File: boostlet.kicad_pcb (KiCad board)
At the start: 2 copper layers, 40 x 35 mm, 53 parts, among them J1 Conn_01x13_Socket, J2 Conn_01x05_Socket, J3 Conn_01x05_Socket, Q1 BSS138, Q2 BSS138, U1 PAM2401, U2 AP2112K-3.3

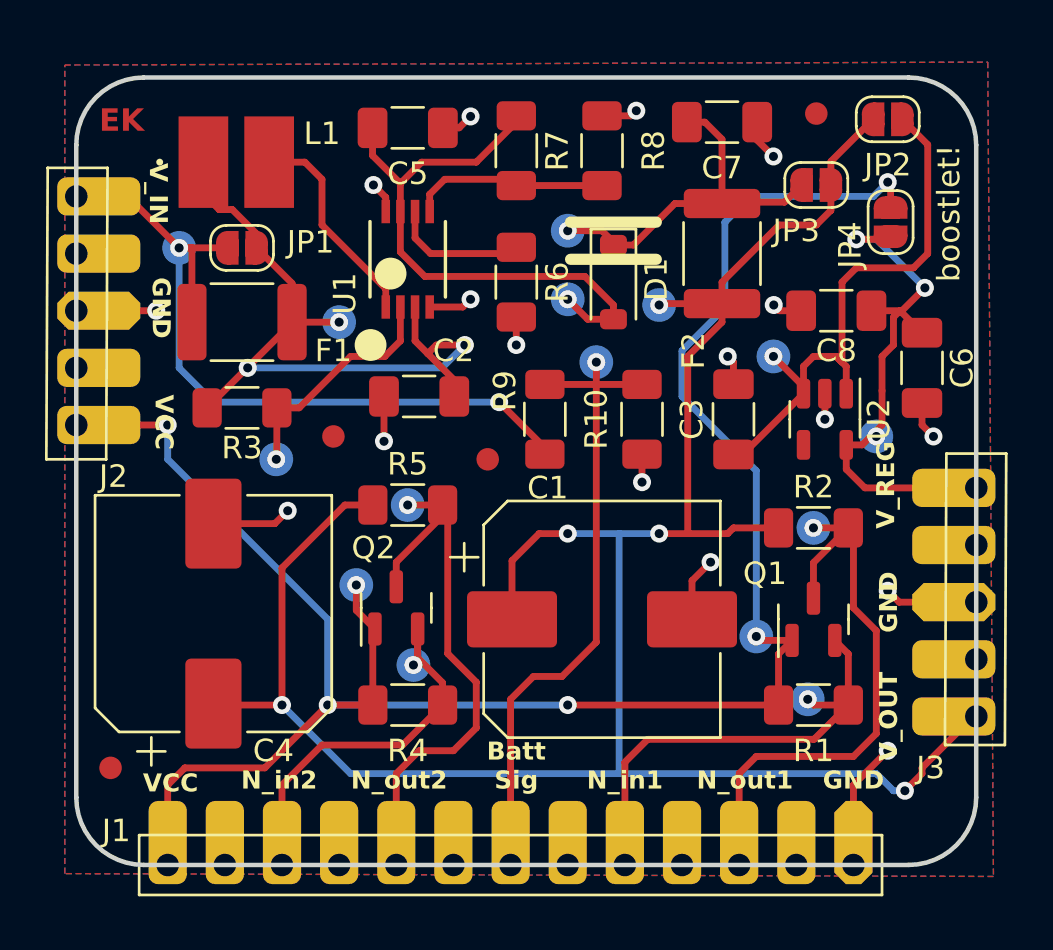
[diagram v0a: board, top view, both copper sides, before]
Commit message: Version 1.2
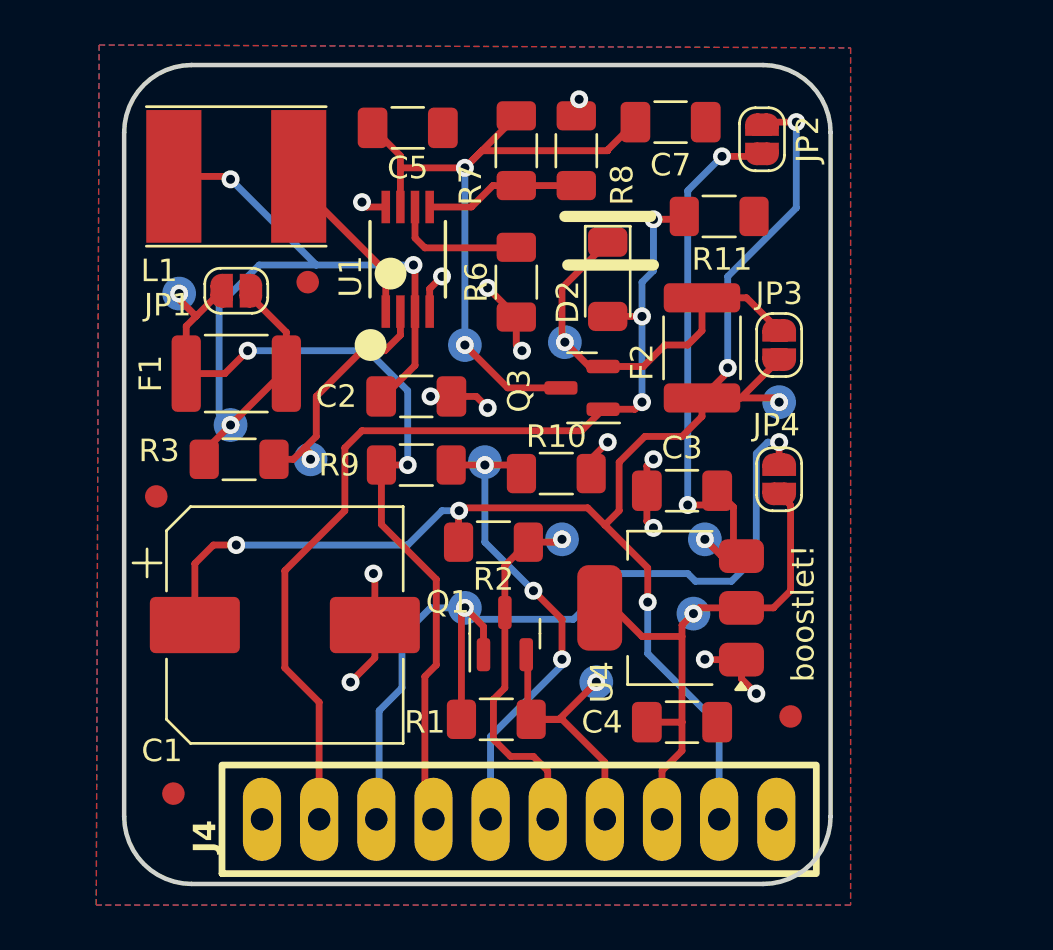
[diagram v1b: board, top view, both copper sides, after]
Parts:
- removed the C4 at (109.7, 103.6)
- removed C6: 4.7 uF, Capacitor_SMD:C_1206_3216Metric_Pad1.33x1.80mm_HandSolder
- removed D1: D_Schottky 3A, Diode_SMD:D_SOD-123
- removed J1: Conn_01x13_Socket, !EK_Library:Castellated_1x13_P2.54mm
- removed J2, J3: Conn_01x05_Socket, !EK_Library:Castellated_1x05_P2.54mm
- removed Q2: BSS138, Package_TO_SOT_SMD:SOT-23
- removed R4, R5: 10k, Resistor_SMD:R_1206_3216Metric_Pad1.30x1.75mm_HandSolder
- removed TP10, TP8, TP9: TestPoint, TestPoint:TestPoint_Pad_D1.5mm
- removed U2: AP2112K-3.3, Package_TO_SOT_SMD:SOT-23-5
- added D2: PMEG40T30ERX 40V 3A, Diode_SMD:D_SOD-123, F.Cu at (127.3, 88.8)
- added J4: Conn_01x10_Socket, !RobotButterfly:Oval_1x10_P2.54mm, F.Cu at (111.9, 112.8)
- added Q3: DMG3415U, Package_TO_SOT_SMD:SOT-23, F.Cu at (126.1, 93.6)
- added R11: 100k, Resistor_SMD:R_1206_3216Metric_Pad1.30x1.75mm_HandSolder, F.Cu at (132.2, 86.0)
- added U4: AP2111H-3.3TRG1, Package_TO_SOT_SMD:SOT-223-3_TabPin2, F.Cu at (130.0, 103.4)
- C1: value 680 uF @ 10 V -> 1000 uF @ 16 V
- C3: value 4.7 uF -> 1 uF
- L1: value 2.2 uH, 3 A -> 4.7 uH, 3 A; footprint !EK_Library:INDUCTOR_IND_IFSC_1515AH_VIS-M -> Inductor_SMD:L_Taiyo-Yuden_NR-60xx_HandSoldering
- moved FID3 26.8 mm to (135.4, 108.2)
- moved C4 19.5 mm to (130.6, 108.5), turned to 0 degrees
- moved FID4 14.8 mm to (107.2, 98.4)
- moved R2 14.2 mm to (122.2, 100.5)
- moved R1 14.1 mm to (122.3, 108.3)
- moved C1 14.1 mm to (112.9, 104.1)
- moved Q1 13.7 mm to (122.7, 104.5)
- moved TP2 13.0 mm to (120.9, 103.4)
- moved JP4 12.5 mm to (134.9, 97.7)
- moved TP13 11.3 mm to (131.1, 103.6)
- moved TP5 11.2 mm to (125.2, 100.3)
- moved TP1 9.43 mm to (126.7, 106.7)
- moved TP11 8.68 mm to (131.6, 100.3)
- moved JP3 7.30 mm to (134.9, 91.7), turned to -90 degrees
- moved FID2 6.95 mm to (113.9, 88.9)
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- renumbered C8 to C4, TP16 to TP15, TP15 to TP16
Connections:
- C5 pad 1: Net-(D1-A) -> /V_BOOST
- C7 pad 1: Net-(D1-K) -> /V_BOOST
- F2 pad 1: Net-(D1-K) -> /5V
- F2 pad 2: /5V -> Net-(D2-K)
- JP3 pad 1: /5V -> Net-(D2-K)
- JP3 pad 2: Net-(D1-K) -> /5V
- R7 pad 1: Net-(D1-A) -> /V_BOOST
- TP12 pad 1: Net-(D1-A) -> /V_BOOST
- TP14 pad 1: Net-(D1-K) -> Net-(D2-K)
- U1 pad 7: Net-(D1-A) -> /V_BOOST
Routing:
- net VCC: track 93.9 -> 41.2 mm, vias 6 -> 2
- net /V_BUS: track 0.00 -> 43.6 mm, vias 0 -> 3
- net /V_BOOST: track 0.00 -> 31.5 mm, vias 0 -> 2
- net /5V: track 99.7 -> 70.5 mm, vias 5 -> 6
- net Net-(D1-A): track 26.1 -> 0.00 mm, vias 1 -> 0
- net /NEO_OUT2: track 25.0 -> 0.00 mm, vias 1 -> 0
- net Net-(D2-K): track 0.00 -> 18.0 mm, vias 0 -> 1
- net /NEO_IN2: track 17.7 -> 0.00 mm, vias 1 -> 0
- net Net-(D1-K): track 16.6 -> 0.00 mm, vias 1 -> 0
- net GND: track 38.1 -> 23.6 mm, vias 17 -> 14
- net /NEO_OUT1: track 25.9 -> 16.1 mm
- net /NEO_IN1: track 20.6 -> 13.1 mm
- net /BATT_SIG: track 29.0 -> 22.1 mm, vias 1 -> 3
- net Net-(JP1-B): track 32.6 -> 39.1 mm
- net /V_BATT: track 34.9 -> 38.3 mm, vias 2 -> 3
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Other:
- board size 40 x 35 mm -> 31.4 x 36.4 mm
- board text added: "--- Populated: ---"
- board text added: "N_in"
- board text added: "N_out"
- board text added: "Neo"
- board text added: "V_BATT"
- board text added: "V_BATT: 0.9-4.75V V_OUT: 5V, 3A V_REG: 3.3V, 0.6A"
- board text added: "V_BUS"
- board text added: "by RobotZwrrl.xyz RobotMissions.org 03-09-24 v1.2"
- board text removed: "2xAA"
- board text removed: "3xAA"
- board text removed: "Batt Sig:"
- board text removed: "EK"
- board text removed: "LiPo 1S"
- board text removed: "N_in1"
- board text removed: "N_in2"
- board text removed: "N_out1"
- board text removed: "N_out2"
- board text removed: "Neo 1"
- board text removed: "Neo 2"
- board text removed: "Other"
- board text removed: "Unpopulated"
- board text removed: "V_IN"
- board text removed: "V_IN: 0.9 - 4.75V V_OUT: 5V, 3A V_REG: 3.3V, 1A"
- board text removed: "by RobotZwrrl.xyz RobotMissions.org 12-30-23 v1.0"
